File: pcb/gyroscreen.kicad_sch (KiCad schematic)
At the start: 26 parts, among them J1 USB C 2.0 Receptacle, J2 AVR-ISP-6, SW1 SW_Push, U1 MCP1703Ax-330xxTT, U2 ATmega32U4-A, U3 MPU-6050, Y1 16MHz Crystal

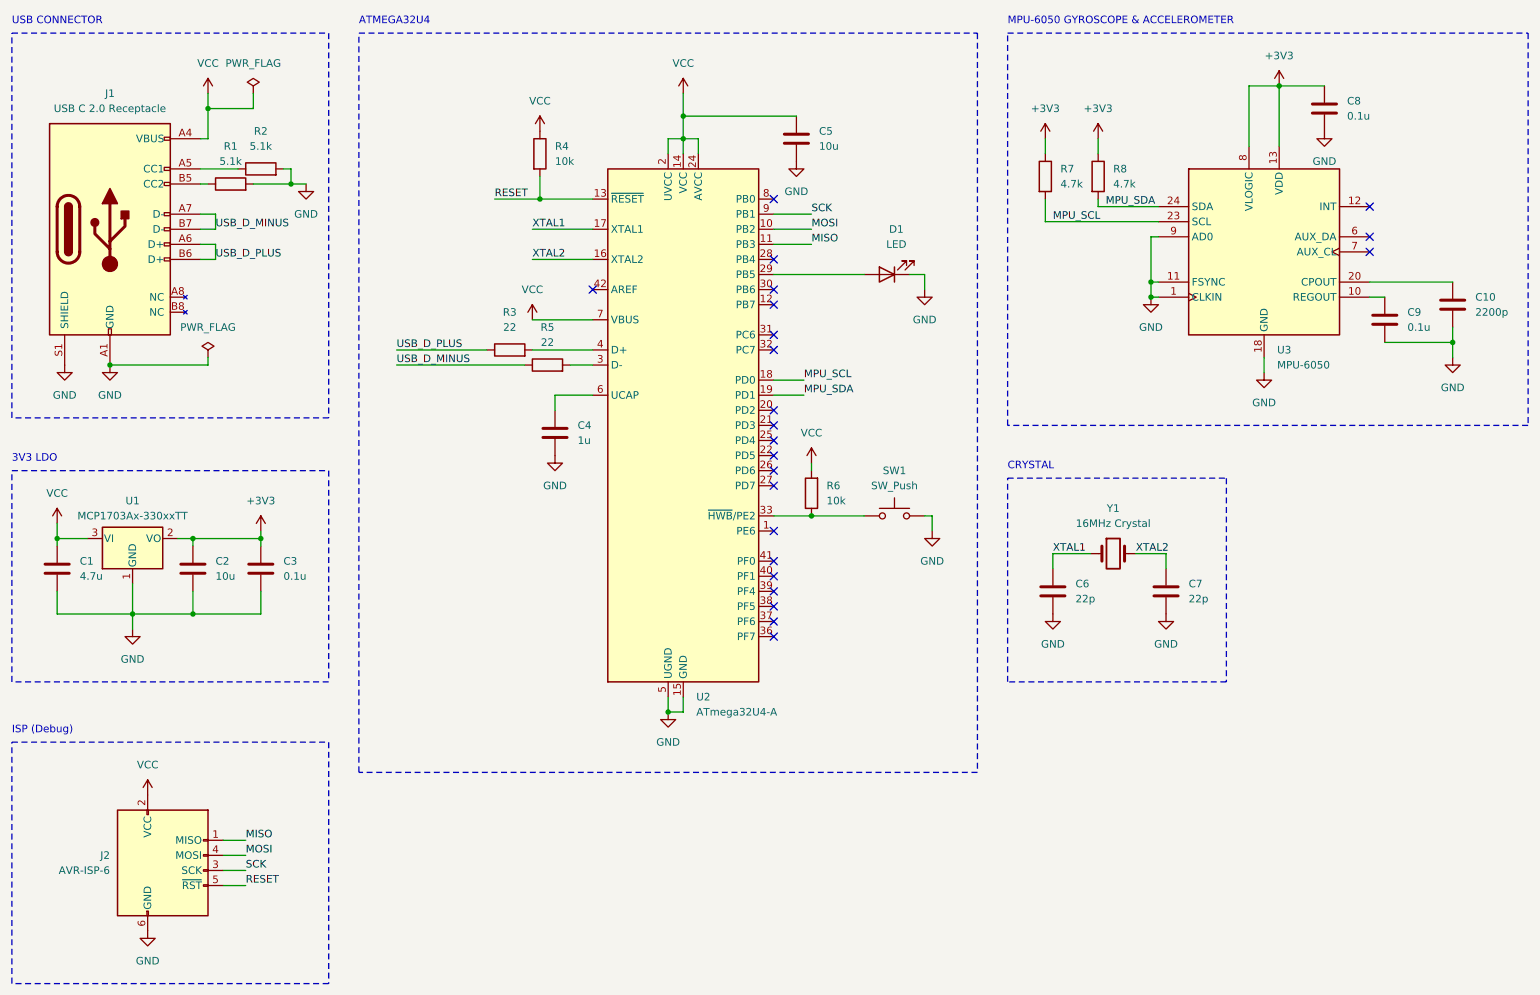
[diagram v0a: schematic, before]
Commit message: Schematic Revision 2
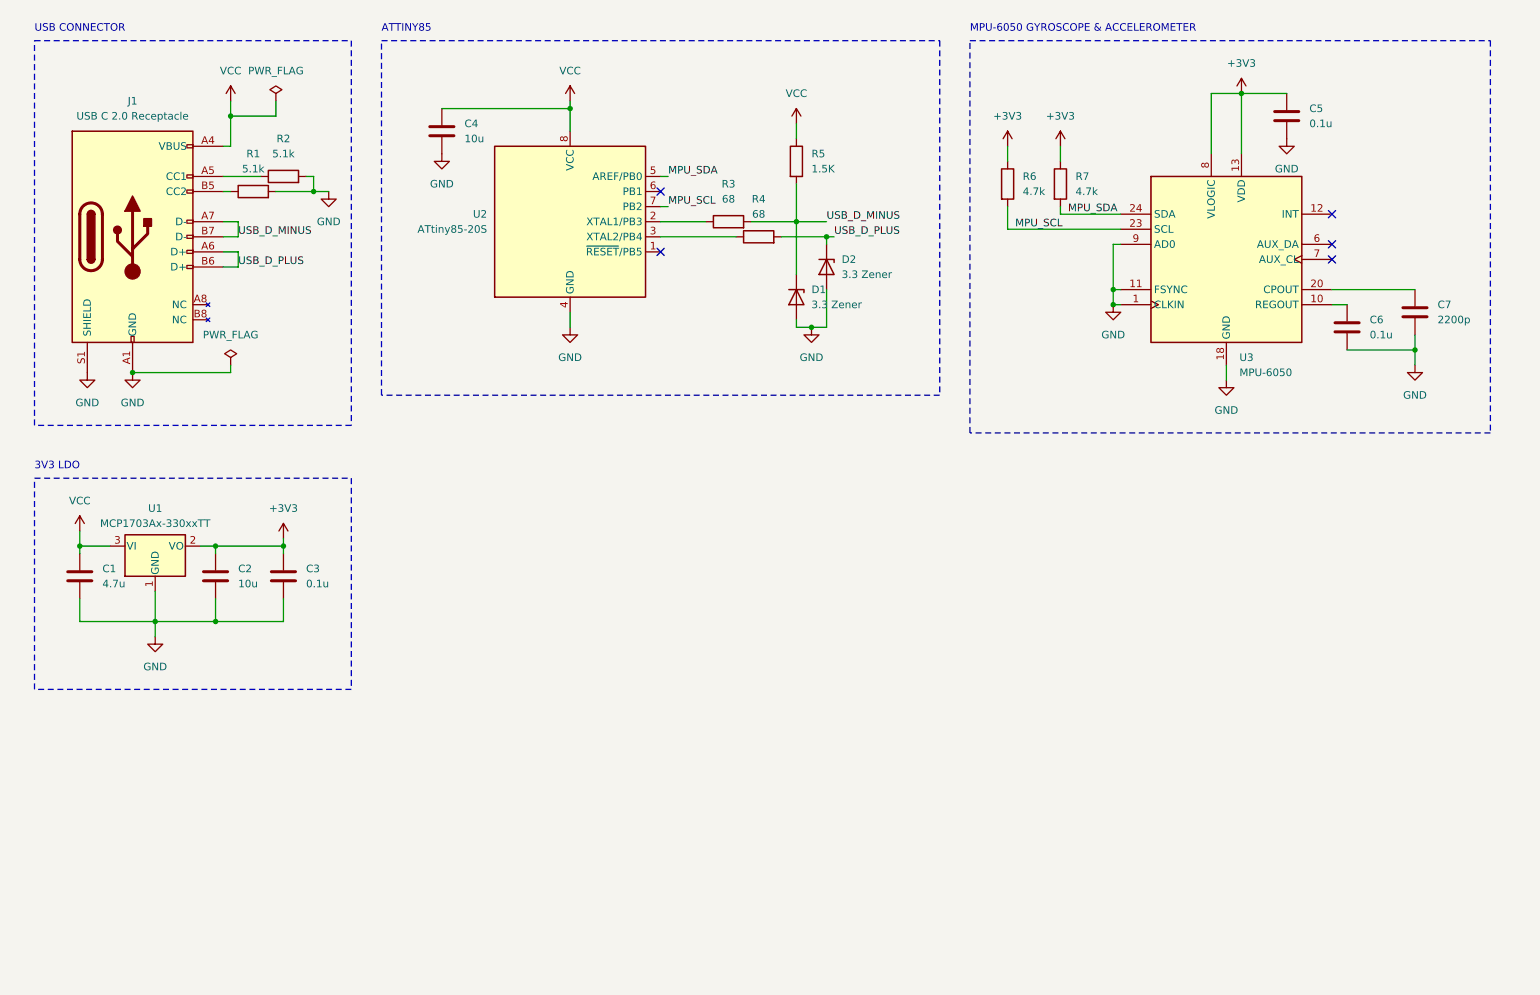
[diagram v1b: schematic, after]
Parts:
- removed C4: 1u, Capacitor_SMD:C_0805_2012Metric_Pad1.18x1.45mm_HandSolder, symbol Device:C
- removed C6, C7: 22p, Capacitor_SMD:C_0805_2012Metric_Pad1.18x1.45mm_HandSolder, symbol Device:C
- removed D1: LED, LED_THT:LED_D1.8mm_W3.3mm_H2.4mm, symbol Device:LED
- removed J2: AVR-ISP-6, Connector_PinHeader_2.54mm:PinHeader_2x03_P2.54mm_Vertical, symbol Connector:AVR-ISP-6
- removed R4, R6: 10k, Resistor_SMD:R_0805_2012Metric_Pad1.20x1.40mm_HandSolder, symbol Device:R
- removed SW1: SW_Push, Button_Switch_SMD:SW_Push_1P1T_NO_6x6mm_H9.5mm, symbol Switch:SW_Push
- removed U2: ATmega32U4-A, Package_QFP:TQFP-44_10x10mm_P0.8mm, symbol MCU_Microchip_ATmega:ATmega32U4-A
- removed Y1: 16MHz Crystal, Crystal:Crystal_SMD_2012-2Pin_2.0x1.2mm, symbol Device:Crystal
- added D1, D2: 3.3 Zener, Diode_SMD:D_0805_2012Metric_Pad1.15x1.40mm_HandSolder, symbol Device:D_Zener
- added R5: 1.5K, Resistor_SMD:R_0805_2012Metric_Pad1.20x1.40mm_HandSolder, symbol Device:R
- added U2: ATtiny85-20S, Package_SO:SOIC-8W_5.3x5.3mm_P1.27mm, symbol MCU_Microchip_ATtiny:ATtiny85-20S
- R3: value 22 -> 68
- R4: renamed from R5; value 22 -> 68
- renumbered C5 to C4, C8 to C5, C9 to C6, C10 to C7, R7 to R6, R8 to R7
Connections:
- net GND: now also D1.2 (A), D2.2 (A), U2.4 (GND)
- net MPU_SCL: now also U2.7 (PB2)
- net MPU_SDA: now also U2.5 (AREF/PB0)
- net USB_D_MINUS: now also R3.2, D1.1 (K), R5.2; no longer R4.1
- net USB_D_PLUS: now also R4.2, D2.1 (K); no longer R3.1
- net VCC: now also R5.1, U2.8 (VCC)
- new net: R4.1, U2.3 (XTAL2/PB4)
- new net: R3.1, U2.2 (XTAL1/PB3)
- no-connect marks 23 -> 5
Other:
- note added: "ATTINY85"
- note removed: "ATMEGA32U4"
- note removed: "CRYSTAL"
- note removed: "ISP (Debug)"
- moved on the sheet: C1, C2, C3, C4, C5, C6, C7, J1, R1, R2, R3, R4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
